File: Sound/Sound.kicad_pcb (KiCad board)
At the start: 4 copper layers, 133.6 x 74.7 mm, 29 parts, among them J1 2x19 2.54mm Right-angled Head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, U1 74HCT74, U3 ATF22V10C, U5 LM386, U6 LM386, U7 LM386

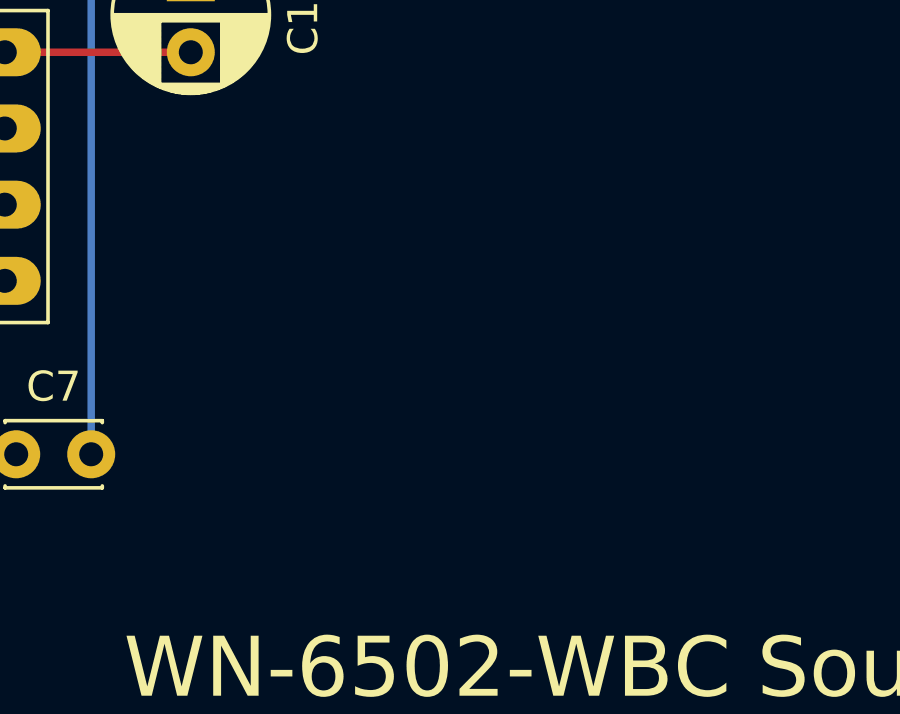
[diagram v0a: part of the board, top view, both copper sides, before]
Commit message: Logo added...
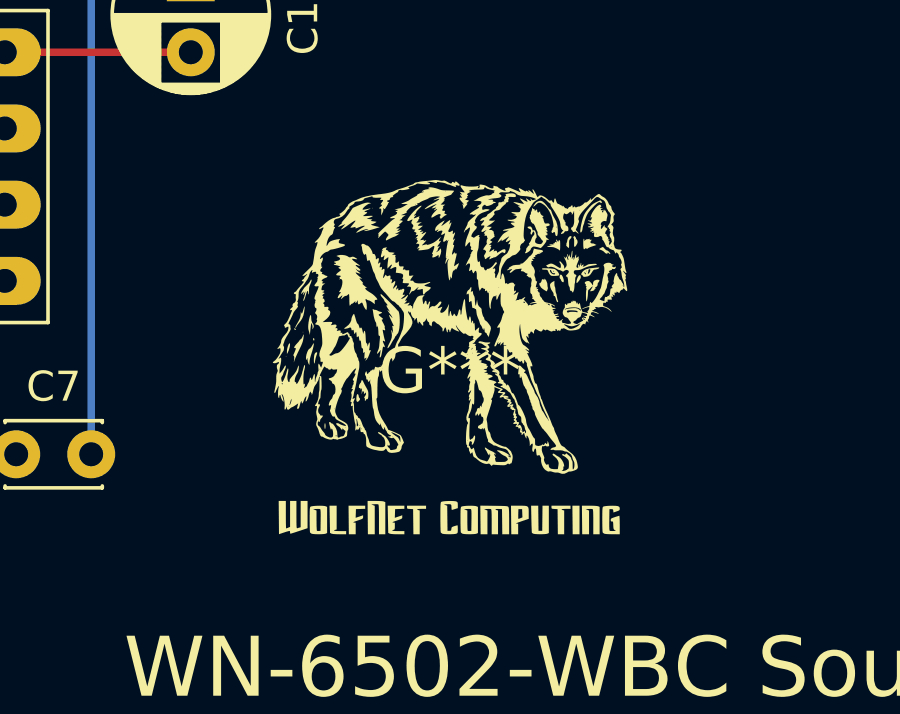
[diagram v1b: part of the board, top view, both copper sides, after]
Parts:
- added G***: LOGO, WolfNet:WolfNet-Logo_silkscreen, F.Cu at (71.1, 81.3)
